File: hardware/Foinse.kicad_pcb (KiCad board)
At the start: 6 copper layers, 60 x 60 mm, 109 parts, among them J1 ESQ-110-X-X-D, J15 39-29-1048, J3 PJ-063AH, J4 5023860570, Q1 IPD90P04P4L04ATMA1, Q2 IPD90P04P4L04ATMA1, U1 STM32F072C8Tx, U17 LTC4412xS6, U19 TPS56A37RPAR, U2 MPM3650CGQW-P, U4 TJA1051T-3, U5 TPS563203, U6 ACS71240KEXBLT-010B3, U7 ACS71240KEXBLT-010B3

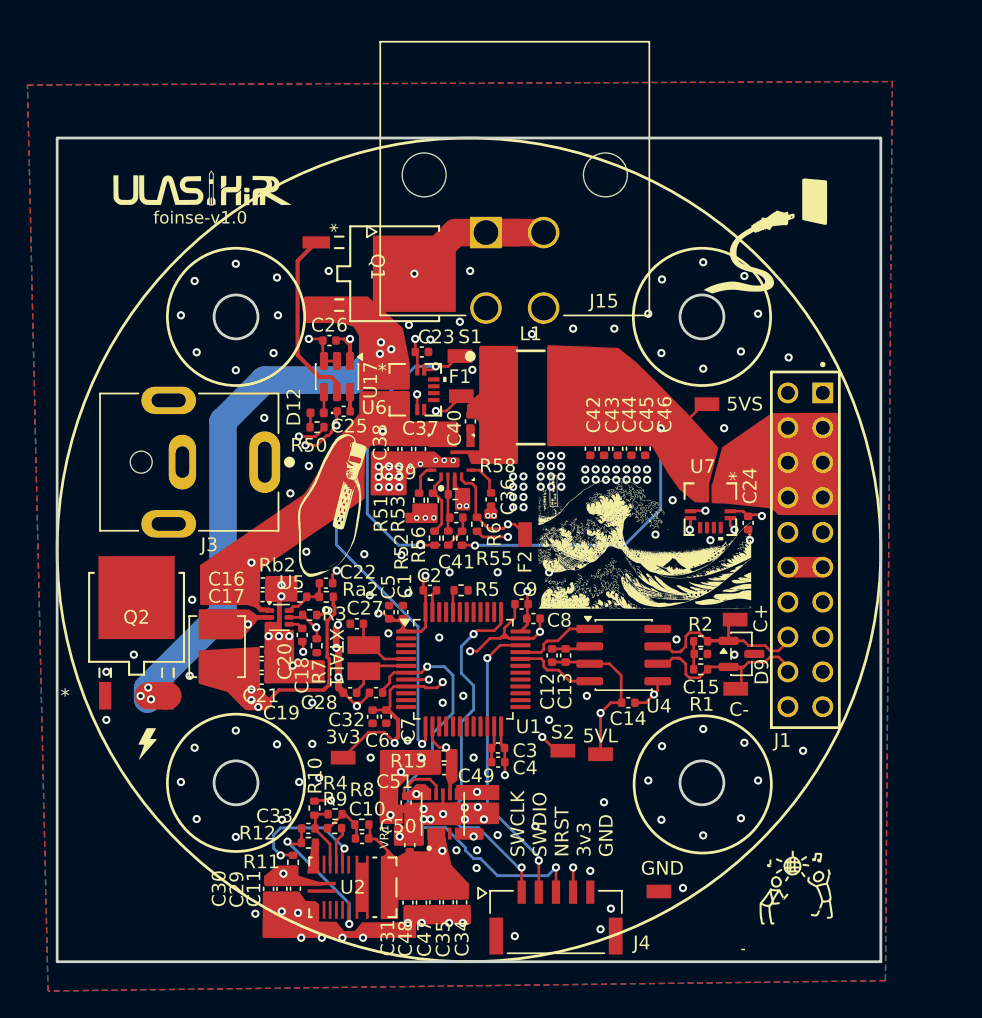
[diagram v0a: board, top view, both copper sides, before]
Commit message: minor changes
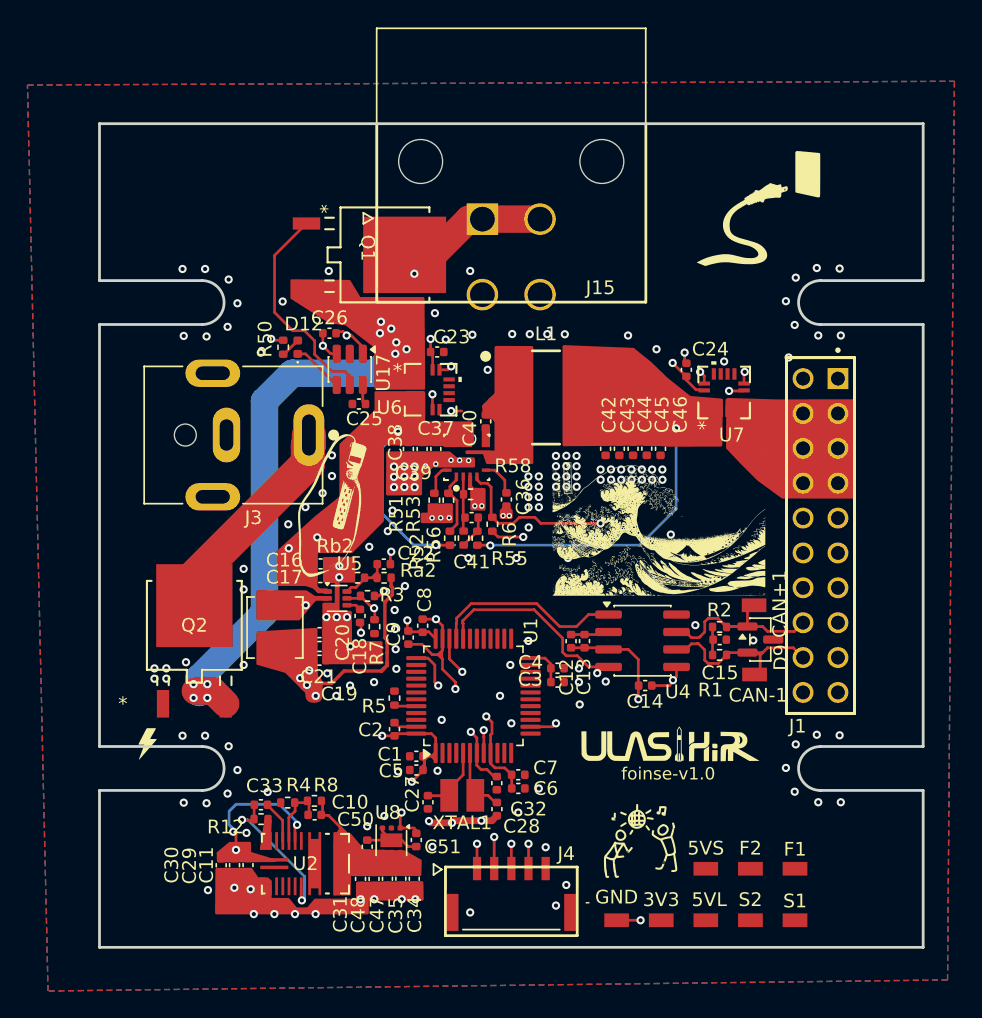
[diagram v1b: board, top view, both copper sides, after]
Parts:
- removed C49: 4.7uf, Capacitor_SMD:C_0402_1005Metric
- removed R10, R9: 0Ω, Resistor_SMD:R_0402_1005Metric
- removed R11: 499kΩ, Resistor_SMD:R_0402_1005Metric
- removed R13: 33.2kΩ, Resistor_SMD:R_0402_1005Metric
- removed VR1: LT3045EDD_PBF, footprints:SON50P300X300X80-11N
- added U8: TLV75533PDRV, Package_SON:WSON-6-1EP_2x2mm_P0.65mm_EP1x1.6mm, F.Cu at (144.3, 102.3)
- 3V3: renamed from 3v3; value S2761-46R -> 3V3
- 5VL: value S2761-46R -> 5vLogic
- C50: value 4.7uf -> 1uf
- C51: value 10uf -> 1uf
- F1: value S2761-46R -> FAULT1
- F2: value S2761-46R -> FAULT2
- GND: value S2761-46R -> GND
- moved G*** 52.9 mm to (165.1, 95.3)
- moved S1 47.8 mm to (173.7, 108.1)
- moved F1 42.1 mm to (173.7, 104.3)
- moved 5VS 33.8 mm to (167.2, 104.3)
- moved F2 29.4 mm to (170.4, 104.3), turned to 180 degrees
- moved 3V3 26.0 mm to (163.9, 108.1)
- moved S2 18.4 mm to (170.4, 108.1), turned to 180 degrees
- moved 5VL 14.3 mm to (167.2, 108.1)
- moved C27 14.0 mm to (146.9, 99.5), turned to 90 degrees
- moved C28 13.6 mm to (151.9, 100.0), turned to -90 degrees
- moved XTAL1 12.3 mm to (149.4, 99.0), turned to 0 degrees
- moved C24 12.0 mm to (165.8, 68.0), turned to -90 degrees
- moved G*** 11.8 mm to (162.4, 102.6)
- moved C6 11.8 mm to (153.5, 98.5), turned to 0 degrees
- moved C5 11.7 mm to (146.1, 97.2), turned to 180 degrees
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- renumbered C+ to CAN+1, C- to CAN-1
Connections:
- C10 pad 2: Net-(C10-Pad2) -> Net-(U2-FB)
- C33 pad 1: AGND -> GND
- R4 pad 1: AGND -> GND
- R4 pad 2: Net-(C10-Pad2) -> Net-(U2-FB)
- R8 pad 1: Net-(C10-Pad2) -> Net-(U2-FB)
- U2 pad 16: Net-(U2-EN) -> 5V_LOGIC
- U2 pad 18: AGND -> GND
- U7 pad 1: 5VSERVO -> 5VSERVO_S
- U7 pad 2: 5VSERVO -> 5VSERVO_S
- U7 pad 3: 5VSERVO_S -> 5VSERVO
- U7 pad 4: 5VSERVO_S -> 5VSERVO
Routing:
- net 3.3V: track 142.9 -> 38.3 mm, vias 12 -> 10
- net Sense1: track 37.8 -> 0.95 mm, vias 2 -> 1
- net NRST: track 33.2 -> 6.46 mm
- net Fault1: track 29.4 -> 4.15 mm
- net SWCLK: track 26.7 -> 4.96 mm
- net 5VLOGIC: track 106.3 -> 84.8 mm, vias 6 -> 7
- net GND: track 41.0 -> 57.3 mm, vias 187 -> 183
- net SWDIO: track 21.4 -> 5.10 mm
- net 5V_LOGIC: track 1.59 -> 11.9 mm, vias 1 -> 3
- net Net-(U2-EN): track 9.96 -> 0.00 mm, vias 2 -> 0
- net CAN_-: track 5.96 -> 14.6 mm, vias 0 -> 1
- net CAN_+: track 5.99 -> 14.1 mm
- net Fault2: track 23.2 -> 29.7 mm
- net AGND: track 5.06 -> 0.00 mm
- net Net-(C10-Pad2): track 3.76 -> 0.00 mm
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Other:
- outline, holes or cut-outs redrawn
